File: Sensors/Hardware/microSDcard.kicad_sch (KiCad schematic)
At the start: 2 parts

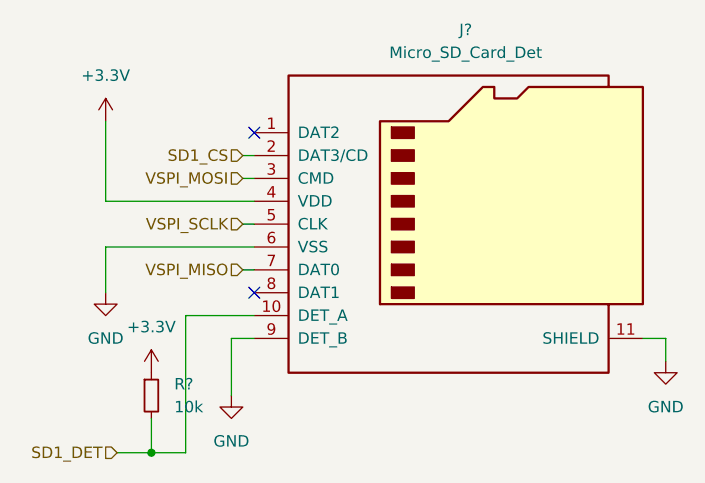
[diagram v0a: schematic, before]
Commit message: fixed hierarchical labels and added ref values
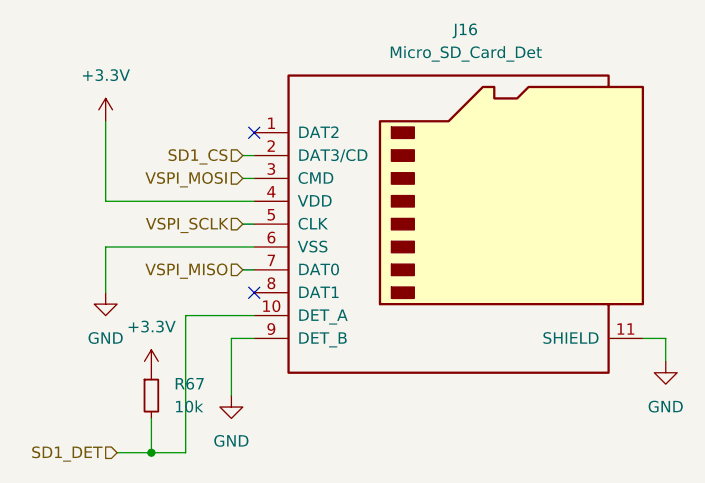
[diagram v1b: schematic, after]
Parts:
- gave numbers to parts that had none: 2
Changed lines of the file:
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@@
   (symbol (lib_id "Device:R_Small") (at 143.51 110.49 0) (unit 1)
     (in_bom yes) (on_board yes) (fields_autoplaced)
-    (property "Reference" "R?" (id 0) (at 146.05 109.2199 0)
+    (property "Reference" "R67" (id 0) (at 146.05 109.2199 0)
       (effects (font (size 1.27 1.27)) (justify left))
     )
@@
   (symbol (lib_id "power:GND") (at 152.4 110.49 0) (unit 1)
     (in_bom yes) (on_board yes) (fields_autoplaced)
-    (property "Reference" "#PWR?" (id 0) (at 152.4 116.84 0)
+    (property "Reference" "#PWR0145" (id 0) (at 152.4 116.84 0)
       (effects (font (size 1.27 1.27)) hide)
     )
@@
   (symbol (lib_id "power:+3.3V") (at 138.43 80.01 0) (unit 1)
     (in_bom yes) (on_board yes) (fields_autoplaced)
-    (property "Reference" "#PWR?" (id 0) (at 138.43 83.82 0)
+    (property "Reference" "#PWR0142" (id 0) (at 138.43 83.82 0)
       (effects (font (size 1.27 1.27)) hide)
     )
@@
   (symbol (lib_id "power:GND") (at 138.43 99.06 0) (unit 1)
     (in_bom yes) (on_board yes) (fields_autoplaced)
-    (property "Reference" "#PWR?" (id 0) (at 138.43 105.41 0)
+    (property "Reference" "#PWR0143" (id 0) (at 138.43 105.41 0)
       (effects (font (size 1.27 1.27)) hide)
     )
@@
   (symbol (lib_id "power:+3.3V") (at 143.51 107.95 0) (unit 1)
     (in_bom yes) (on_board yes) (fields_autoplaced)
-    (property "Reference" "#PWR?" (id 0) (at 143.51 111.76 0)
+    (property "Reference" "#PWR0144" (id 0) (at 143.51 111.76 0)
       (effects (font (size 1.27 1.27)) hide)
     )
@@
   (symbol (lib_id "power:GND") (at 200.66 106.68 0) (unit 1)
     (in_bom yes) (on_board yes) (fields_autoplaced)
-    (property "Reference" "#PWR?" (id 0) (at 200.66 113.03 0)
+    (property "Reference" "#PWR0146" (id 0) (at 200.66 113.03 0)
       (effects (font (size 1.27 1.27)) hide)
     )
@@
   (symbol (lib_id "Connector:Micro_SD_Card_Det") (at 177.8 91.44 0) (unit 1)
     (in_bom yes) (on_board yes) (fields_autoplaced)
-    (property "Reference" "J?" (id 0) (at 178.435 69.85 0))
+    (property "Reference" "J16" (id 0) (at 178.435 69.85 0))
     (property "Value" "Micro_SD_Card_Det" (id 1) (at 178.435 72.39 0))
     (property "Footprint" "Connector_Card:microSD_HC_Hirose_DM3AT-SF-PEJM5" (id 2) (at 229.87 73.66 0)

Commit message: added 10V rail, moved to boosts sheet
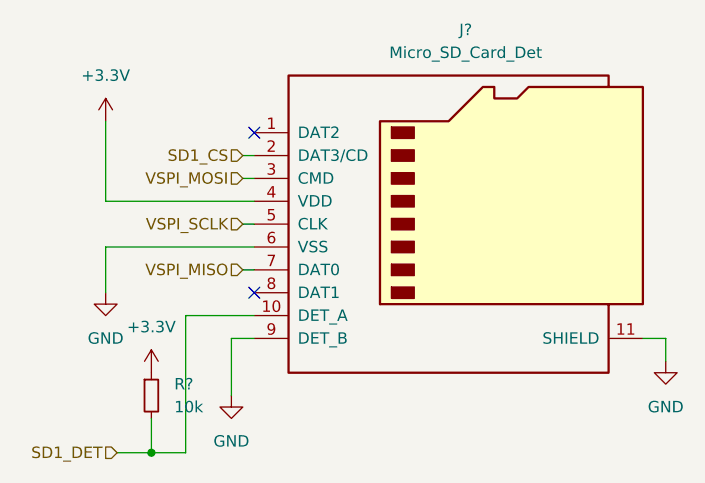
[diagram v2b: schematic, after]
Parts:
- renumbered J16 to J?, R67 to R?
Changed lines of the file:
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@@
   (symbol (lib_id "Device:R_Small") (at 143.51 110.49 0) (unit 1)
     (in_bom yes) (on_board yes) (fields_autoplaced)
-    (property "Reference" "R67" (id 0) (at 146.05 109.2199 0)
+    (property "Reference" "R?" (id 0) (at 146.05 109.2199 0)
       (effects (font (size 1.27 1.27)) (justify left))
     )
@@
   (symbol (lib_id "power:GND") (at 152.4 110.49 0) (unit 1)
     (in_bom yes) (on_board yes) (fields_autoplaced)
-    (property "Reference" "#PWR0145" (id 0) (at 152.4 116.84 0)
+    (property "Reference" "#PWR?" (id 0) (at 152.4 116.84 0)
       (effects (font (size 1.27 1.27)) hide)
     )
@@
   (symbol (lib_id "power:+3.3V") (at 138.43 80.01 0) (unit 1)
     (in_bom yes) (on_board yes) (fields_autoplaced)
-    (property "Reference" "#PWR0142" (id 0) (at 138.43 83.82 0)
+    (property "Reference" "#PWR?" (id 0) (at 138.43 83.82 0)
       (effects (font (size 1.27 1.27)) hide)
     )
@@
   (symbol (lib_id "power:GND") (at 138.43 99.06 0) (unit 1)
     (in_bom yes) (on_board yes) (fields_autoplaced)
-    (property "Reference" "#PWR0143" (id 0) (at 138.43 105.41 0)
+    (property "Reference" "#PWR?" (id 0) (at 138.43 105.41 0)
       (effects (font (size 1.27 1.27)) hide)
     )
@@
   (symbol (lib_id "power:+3.3V") (at 143.51 107.95 0) (unit 1)
     (in_bom yes) (on_board yes) (fields_autoplaced)
-    (property "Reference" "#PWR0144" (id 0) (at 143.51 111.76 0)
+    (property "Reference" "#PWR?" (id 0) (at 143.51 111.76 0)
       (effects (font (size 1.27 1.27)) hide)
     )
@@
   (symbol (lib_id "power:GND") (at 200.66 106.68 0) (unit 1)
     (in_bom yes) (on_board yes) (fields_autoplaced)
-    (property "Reference" "#PWR0146" (id 0) (at 200.66 113.03 0)
+    (property "Reference" "#PWR?" (id 0) (at 200.66 113.03 0)
       (effects (font (size 1.27 1.27)) hide)
     )
@@
   (symbol (lib_id "Connector:Micro_SD_Card_Det") (at 177.8 91.44 0) (unit 1)
     (in_bom yes) (on_board yes) (fields_autoplaced)
-    (property "Reference" "J16" (id 0) (at 178.435 69.85 0))
+    (property "Reference" "J?" (id 0) (at 178.435 69.85 0))
     (property "Value" "Micro_SD_Card_Det" (id 1) (at 178.435 72.39 0))
     (property "Footprint" "Connector_Card:microSD_HC_Hirose_DM3AT-SF-PEJM5" (id 2) (at 229.87 73.66 0)
